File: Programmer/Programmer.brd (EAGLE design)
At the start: 49.5 x 55.9 mm, 33 parts, among them Q2 16Mhz, U1 ATTINY84, X2 C-GRID-04-70543, X3 C-GRID-04-70543

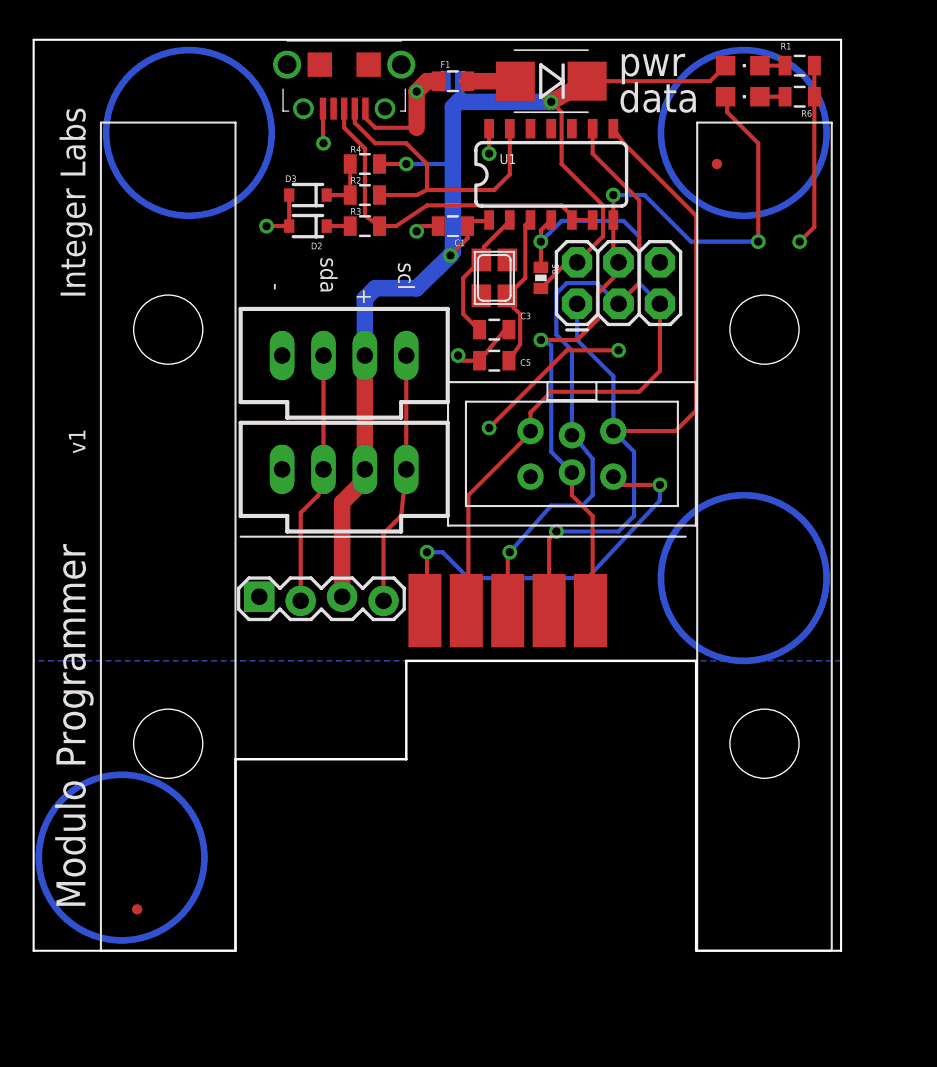
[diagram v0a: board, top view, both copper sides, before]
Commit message: various minor changes
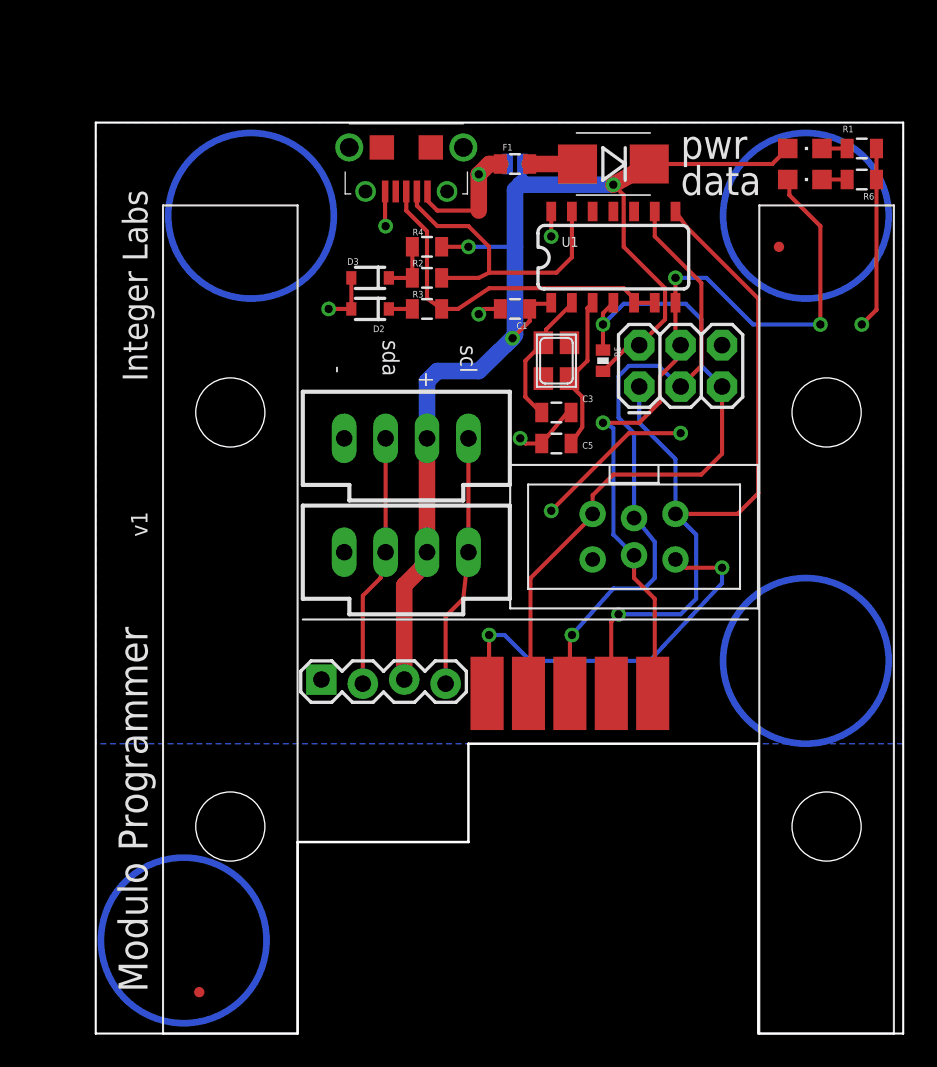
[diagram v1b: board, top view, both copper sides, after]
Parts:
- moved LED1 6.35 mm to (43.5, 54.3)
- moved R1 6.35 mm to (47.0, 54.3)
- moved D3 6.35 mm to (16.8, 46.4)
- moved R2 6.35 mm to (20.3, 46.4)
- moved R4 6.35 mm to (20.3, 48.3)
- moved ICSP 6.35 mm to (33.0, 30.5)
- moved U$1 6.35 mm to (31.6, 22.9)
- moved U$5 6.35 mm to (44.8, 25.4)
- moved JP10 6.35 mm to (41.9, 48.3)
- moved JP11 6.35 mm to (13.8, 21.6)
- moved U$4 6.35 mm to (8.26, 25.4)
- moved X3 6.35 mm to (19.1, 29.5)
- moved C1 6.35 mm to (25.7, 44.5)
- moved F1 6.35 mm to (25.7, 53.3)
- moved JP1 6.35 mm to (25.7, 53.3)
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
